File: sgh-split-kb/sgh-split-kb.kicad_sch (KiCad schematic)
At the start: 29 parts, among them U1 Elite-C

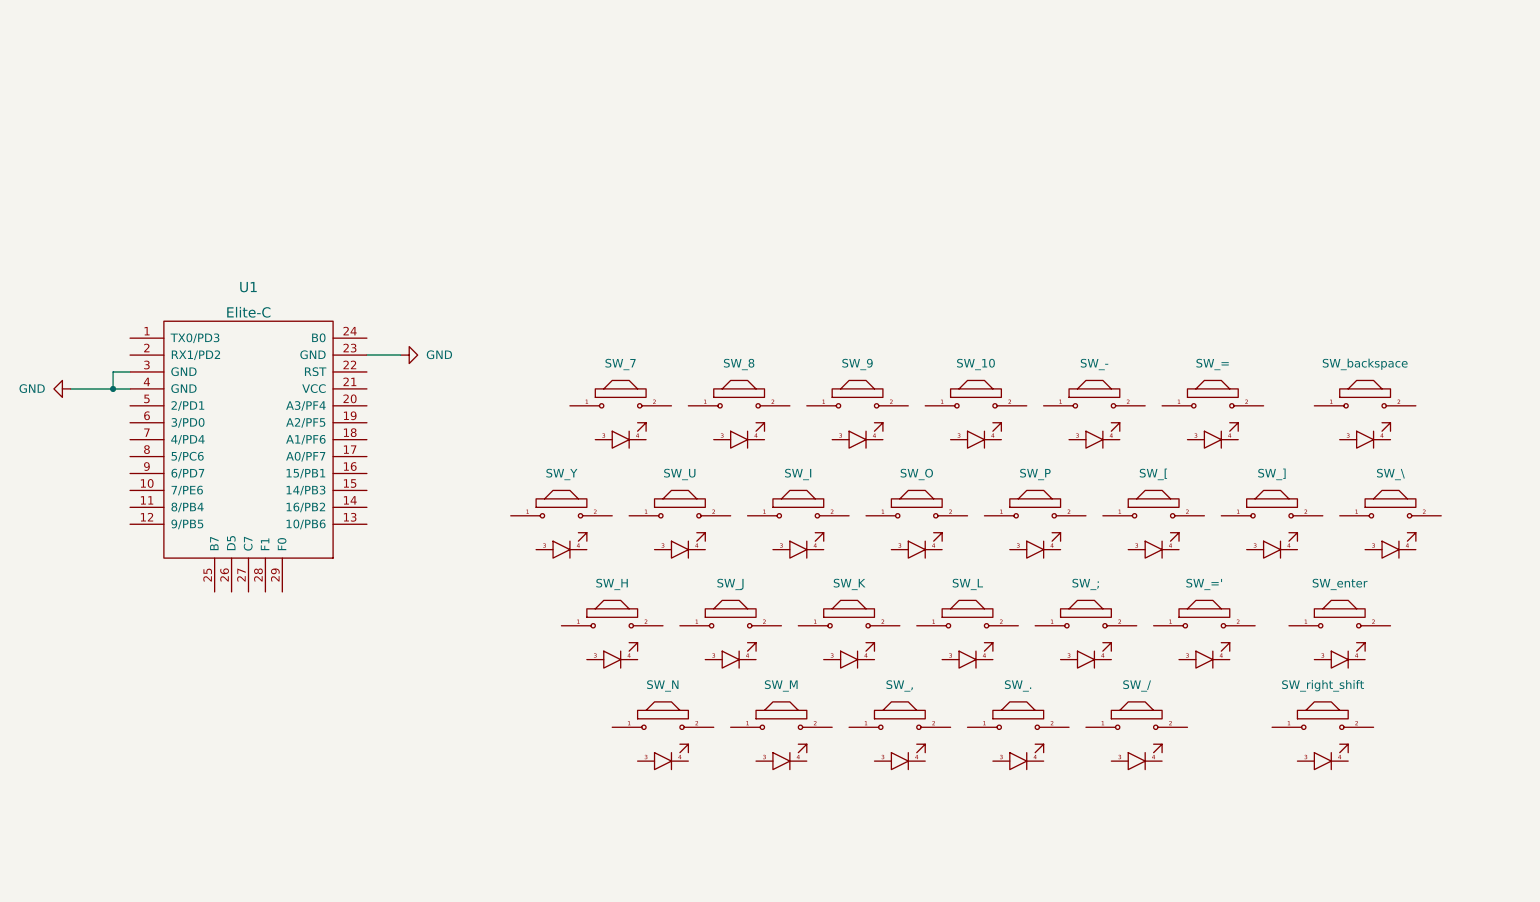
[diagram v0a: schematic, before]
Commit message: basic schematic
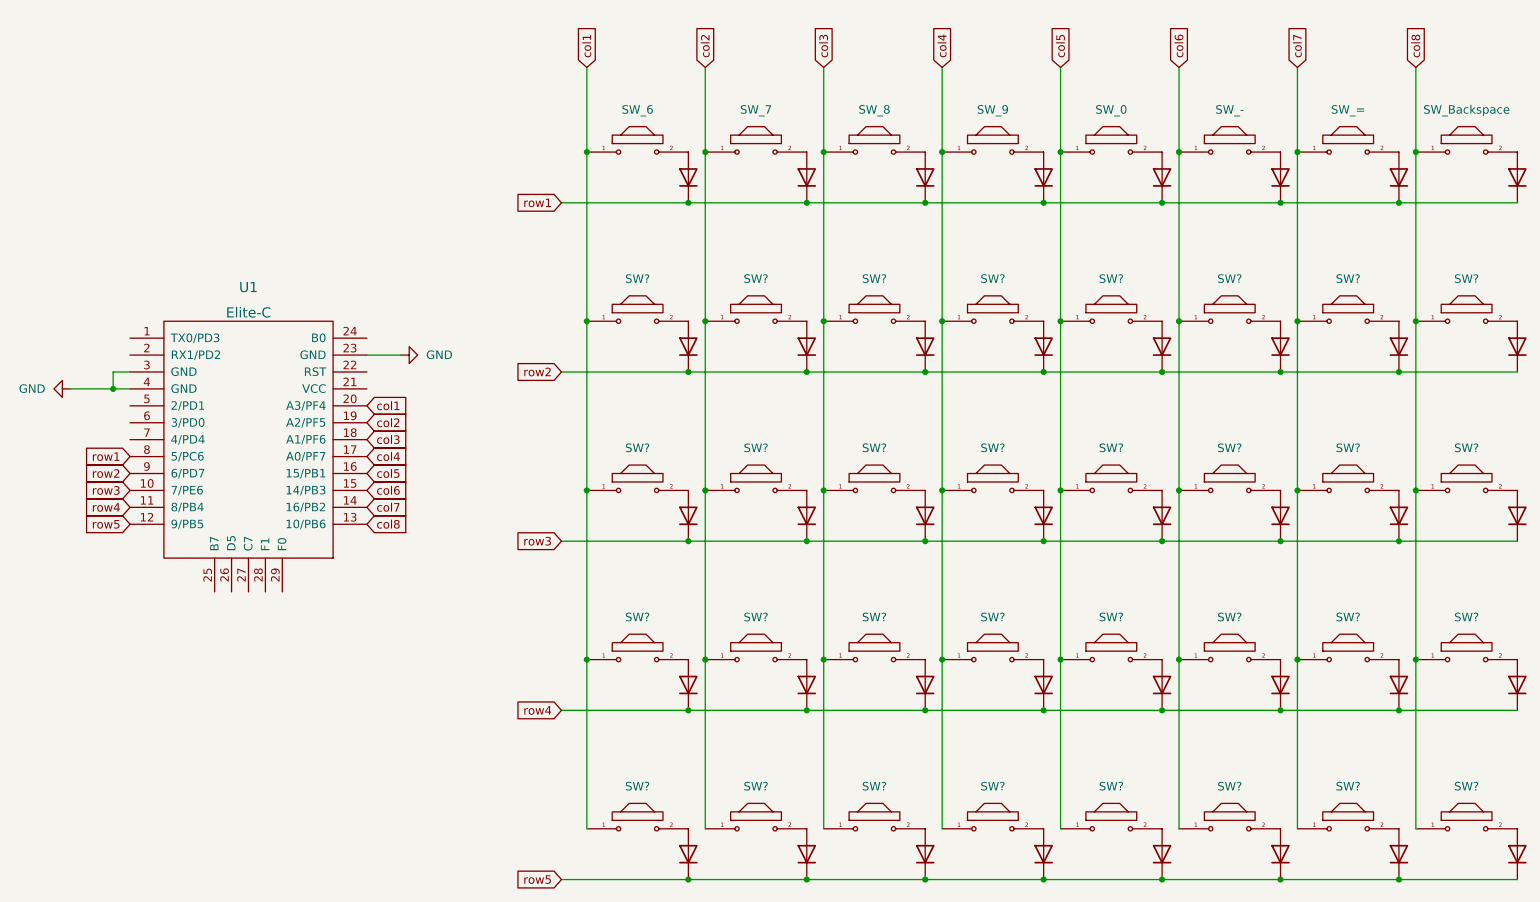
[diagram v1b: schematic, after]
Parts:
- removed SW_,, SW_., SW_/, SW_10, SW_;, SW_=', SW_H, SW_I, SW_J, SW_K, SW_L, SW_M, SW_N, SW_O, SW_P, SW_U, SW_Y, SW_[, SW_\, SW_], SW_backspace, SW_enter, SW_right_shift: MX, keebio:Kailh-PG1350-1u, symbol keebio:MX
- added D? (x40): 1N4148, Diode_THT:D_DO-35_SOD27_P7.62mm_Horizontal, symbol Diode:1N4148
- added SW? (x32), SW_0, SW_6, SW_Backspace: MX, symbol keebio:MX
- SW_-, SW_7, SW_8, SW_9, SW_=: footprint keebio:Kailh-PG1350-1u -> (none)
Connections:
- net col7: now reaches SW_=.1
- net col7: now also U1.14 (16/PB2), SW?.1, SW?.1, SW?.1, SW?.1
- net at SW_=.2: now also D?.2 (A)
- net col6: now reaches SW_-.1
- net col6: now also U1.15 (14/PB3), SW?.1, SW?.1, SW?.1, SW?.1
- net at SW_-.2: now also D?.2 (A)
- net col4: now reaches SW_9.1
- net col4: now also U1.17 (A0/PF7), SW?.1, SW?.1, SW?.1, SW?.1
- net at SW_9.2: now also D?.2 (A)
- net row3: now reaches U1.10 (7/PE6)
- net row3: now also D?.1 (K), D?.1 (K), D?.1 (K), D?.1 (K), D?.1 (K), D?.1 (K), D?.1 (K), D?.1 (K)
- net row4: now reaches U1.11 (8/PB4)
- net row4: now also D?.1 (K), D?.1 (K), D?.1 (K), D?.1 (K), D?.1 (K), D?.1 (K), D?.1 (K), D?.1 (K)
- net row5: now reaches U1.12 (9/PB5)
- net row5: now also D?.1 (K), D?.1 (K), D?.1 (K), D?.1 (K), D?.1 (K), D?.1 (K), D?.1 (K), D?.1 (K)
- net col8: now reaches U1.13 (10/PB6)
- net col8: now also SW?.1, SW?.1, SW?.1, SW?.1, SW_Backspace.1
- net col5: now reaches U1.16 (15/PB1)
- net col5: now also SW?.1, SW?.1, SW?.1, SW?.1, SW_0.1
- net col3: now reaches U1.18 (A1/PF6)
- net col3: now also SW_8.1, SW?.1, SW?.1, SW?.1, SW?.1
- net col2: now reaches U1.19 (A2/PF5)
- net col2: now also SW_7.1, SW?.1, SW?.1, SW?.1, SW?.1
- net col1: now reaches U1.20 (A3/PF4)
- net col1: now also SW?.1, SW?.1, SW?.1, SW?.1, SW_6.1
- net row1: now reaches U1.8 (5/PC6)
- net row1: now also D?.1 (K), D?.1 (K), D?.1 (K), D?.1 (K), D?.1 (K), D?.1 (K), D?.1 (K), D?.1 (K)
- net row2: now reaches U1.9 (6/PD7)
- net row2: now also D?.1 (K), D?.1 (K), D?.1 (K), D?.1 (K), D?.1 (K), D?.1 (K), D?.1 (K), D?.1 (K)
- net at SW_8.2: now also D?.2 (A)
- net at SW_7.2: now also D?.2 (A)
- new net: D?.2 (A), SW?.2 (x32)
- new net: D?.2 (A), SW_6.2
- new net: D?.2 (A), SW_0.2
- new net: D?.2 (A), SW_Backspace.2
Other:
- title: placeholder title -> sgh-split-kb
